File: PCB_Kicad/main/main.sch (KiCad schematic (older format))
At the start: 21 parts, among them Q1 Q_NMOS_GDS, Q2 Q_NMOS_GDS, U1 LTC3854EMSEPBF, U2 ACS70331EESATR-005U3

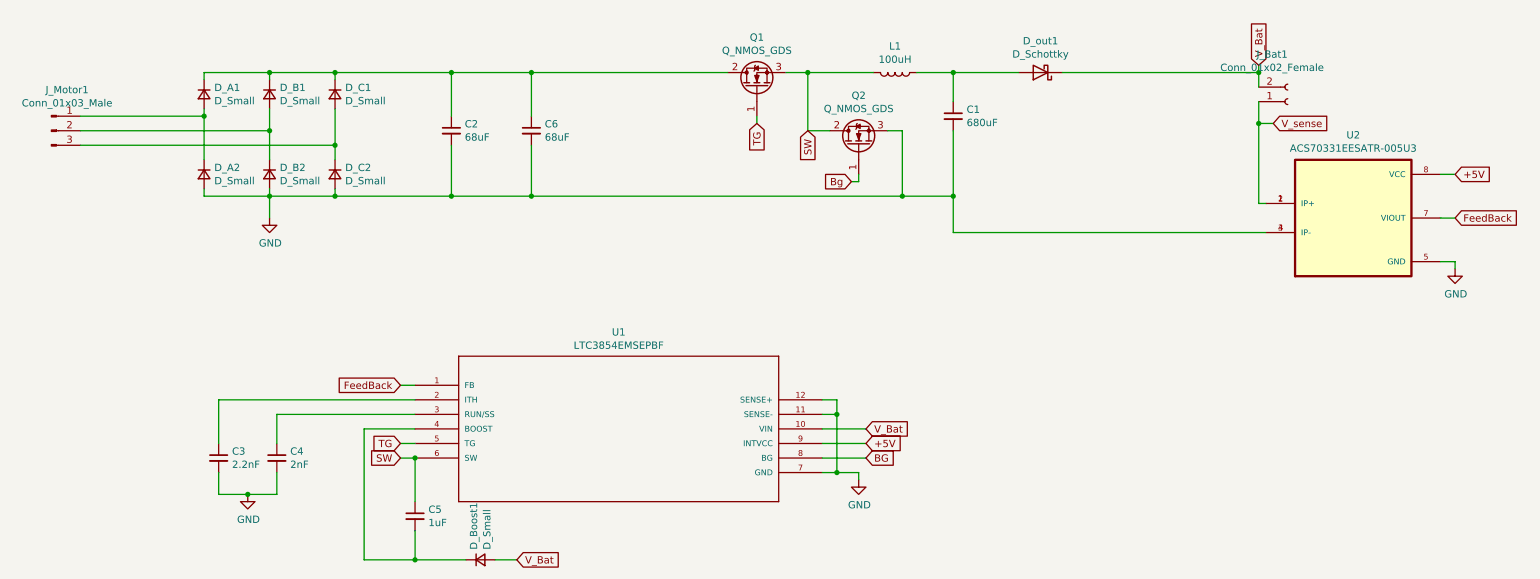
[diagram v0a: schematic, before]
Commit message: kicad update
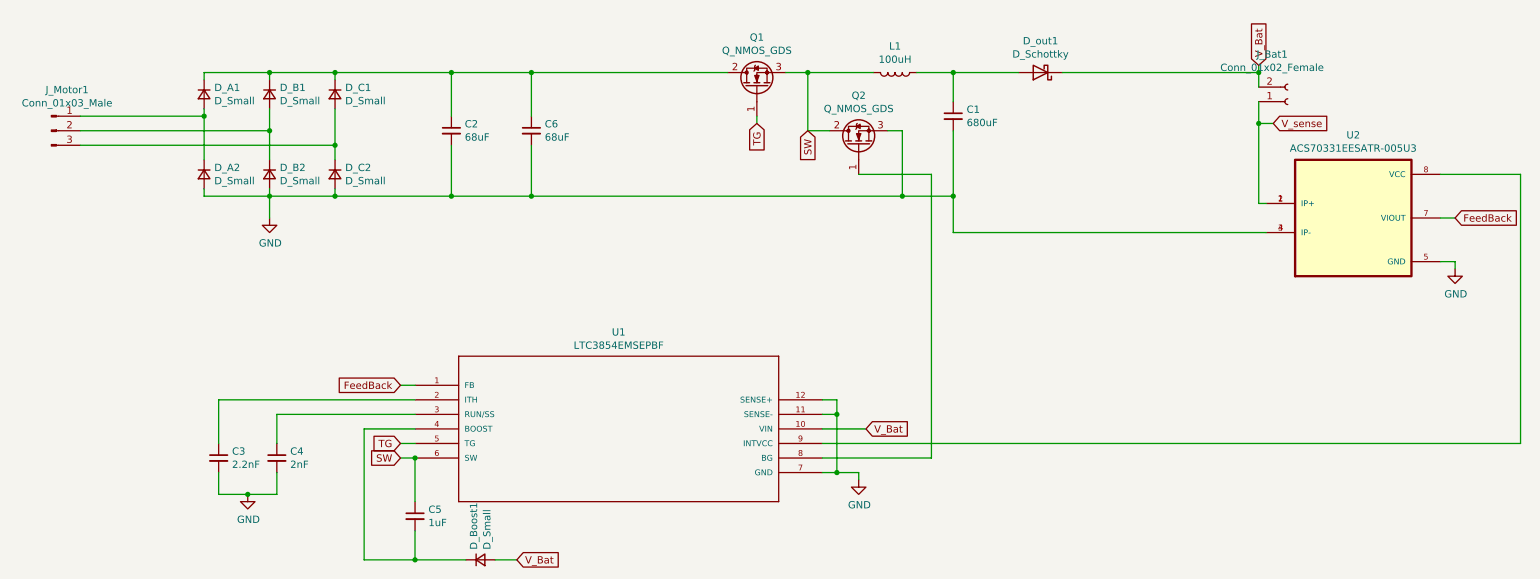
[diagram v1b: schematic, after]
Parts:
- L1: footprint Inductor_THT:L_Radial_D14.2mm_P10.00mm_Neosid_SD14 -> Inductor_SMD:L_Wuerth_HCM-1390
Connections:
- net Bg is gone; now on an unnamed net: Q2.1 (G)
- net +5V: no longer names the net of U1.9 (INTVCC), U2.8 (VCC)
- net BG: no longer names the net of U1.8 (BG)
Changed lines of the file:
@@
 F 0 "L1" V 6519 850 50  0000 C CNN
 F 1 "100uH" V 6610 850 50  0000 C CNN
-F 2 "Inductor_THT:L_Radial_D14.2mm_P10.00mm_Neosid_SD14" H 6700 850 50  0001 C CNN
+F 2 "Inductor_SMD:L_Wuerth_HCM-1390" H 6700 850 50  0001 C CNN
 F 3 "~" H 6700 850 50  0001 C CNN
 	1    6700 850
@@
 Wire Wire Line
 	10550 2150 10450 2150
-Text GLabel 10550 1550 2    50   Input ~ 0
-+5V
-Wire Wire Line
-	10450 1550 10550 1550
-Text GLabel 6500 3400 2    50   Input ~ 0
-+5V
 $Comp
 L power:GND #PWR0102
@@
 	6450 3650 6450 3600
 Wire Wire Line
-	6200 3400 6500 3400
-Wire Wire Line
 	6200 3100 6300 3100
 Wire Wire Line
@@
 Wire Wire Line
 	6500 3300 6200 3300
-Text GLabel 6500 3500 2    50   Input ~ 0
-BG
-Wire Wire Line
-	6200 3500 6500 3500
 Text GLabel 3300 3500 0    50   Input ~ 0
 SW
@@
 Wire Wire Line
 	5750 1150 5750 1200
-Text GLabel 6400 1600 0    50   Input ~ 0
-Bg
-Wire Wire Line
-	6400 1600 6450 1600
-Wire Wire Line
-	6450 1600 6450 1550
 Text GLabel 6100 1250 3    50   Input ~ 0
 SW
@@
 Wire Wire Line
 	4200 1700 6750 1700
+Wire Wire Line
+	6200 3500 6950 3500
+Wire Wire Line
+	6950 3500 6950 1550
+Wire Wire Line
+	6950 1550 6450 1550
+Wire Wire Line
+	11000 1550 11000 3400
+Wire Wire Line
+	11000 3400 6200 3400
+Wire Wire Line
+	10450 1550 11000 1550
 $EndSCHEMATC

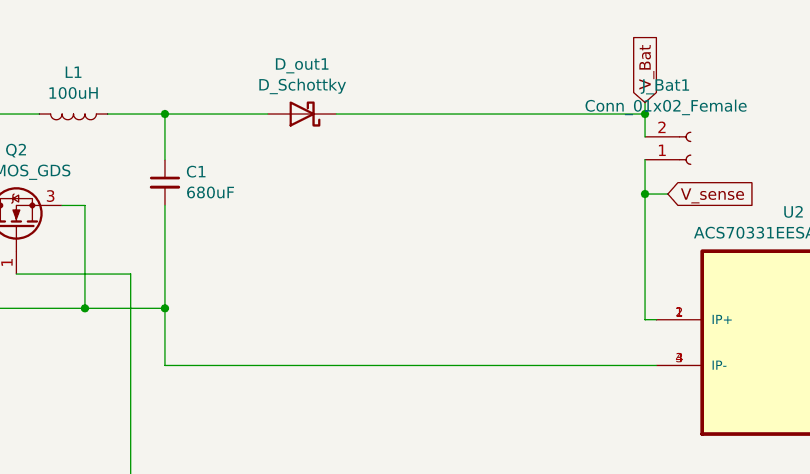
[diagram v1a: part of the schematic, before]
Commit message: model update
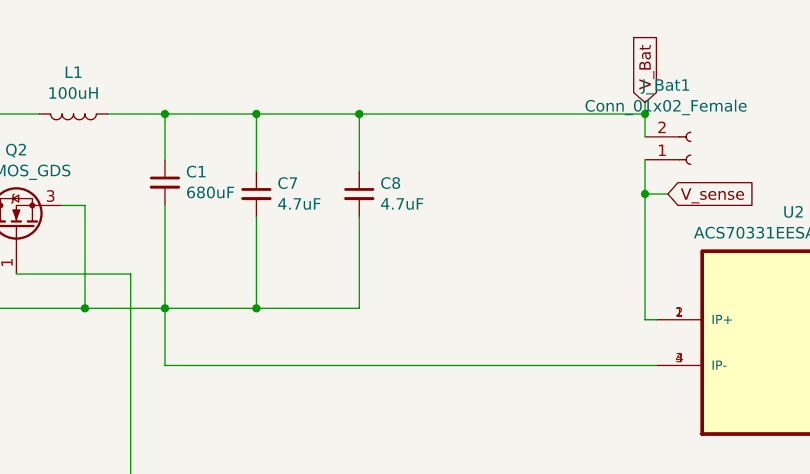
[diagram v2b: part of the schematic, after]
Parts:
- removed D_out1: D_Schottky, Diode_SMD:D_SMB, symbol Device:D_Schottky
- added C7, C8: 4.7uF, Capacitor_SMD:C_2225_5664Metric_Pad1.80x6.60mm_HandSolder, symbol Device:C_Small
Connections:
- net GND: now also C7.2, C8.2
- net V_Bat: now also C1.1, L1.1, C7.1, C8.1
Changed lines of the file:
@@
 Connection ~ 7100 850
 Wire Wire Line
-	7100 850  7550 850
+	7100 850  7500 850
 Wire Wire Line
 	7100 850  7100 1050
@@
 	9200 950  9200 850
 Wire Wire Line
-	9200 850  7850 850
-Wire Wire Line
 	9200 1050 9200 1200
 Text GLabel 9300 1200 2    50   Input ~ 0
@@
 	9200 850  9200 800
 Connection ~ 9200 850
-$Comp
-L Device:D_Schottky D_out1
-U 1 1 6006BA40
-P 7700 850
-F 0 "D_out1" H 7700 633 50  0000 C CNN
-F 1 "D_Schottky" H 7700 724 50  0000 C CNN
-F 2 "Diode_SMD:D_SMB" H 7700 850 50  0001 C CNN
-F 3 "~" H 7700 850 50  0001 C CNN
-	1    7700 850
-	-1   0    0    1
-$EndComp
 $Comp
 L power:GND #PWR0112
@@
 Wire Wire Line
 	10450 1550 11000 1550
+$Comp
+L Device:C_Small C7
+U 1 1 5FFE17AF
+P 7500 1200
+F 0 "C7" H 7592 1246 50  0000 L CNN
+F 1 "4.7uF" H 7592 1155 50  0000 L CNN
+F 2 "Capacitor_SMD:C_2225_5664Metric_Pad1.80x6.60mm_HandSolder" H 7500 1200 50  0001 C CNN
+F 3 "~" H 7500 1200 50  0001 C CNN
+	1    7500 1200
+	1    0    0    -1
+$EndComp
+Wire Wire Line
+	7500 1100 7500 850
+Connection ~ 7500 850
+Wire Wire Line
+	7500 1300 7500 1700
+Wire Wire Line
+	7500 1700 7100 1700
+Wire Wire Line
+	7500 850  7950 850
+Wire Wire Line
+	7950 1100 7950 850
+Connection ~ 7950 850
+Wire Wire Line
+	7950 1300 7950 1700
+Wire Wire Line
+	7950 1700 7500 1700
+Connection ~ 7500 1700
+$Comp
+L Device:C_Small C8
+U 1 1 5FFE1E1F
+P 7950 1200
+F 0 "C8" H 8042 1246 50  0000 L CNN
+F 1 "4.7uF" H 8042 1155 50  0000 L CNN
+F 2 "Capacitor_SMD:C_2225_5664Metric_Pad1.80x6.60mm_HandSolder" H 7950 1200 50  0001 C CNN
+F 3 "~" H 7950 1200 50  0001 C CNN
+	1    7950 1200
+	1    0    0    -1
+$EndComp
+Wire Wire Line
+	7950 850  9200 850
 $EndSCHEMATC

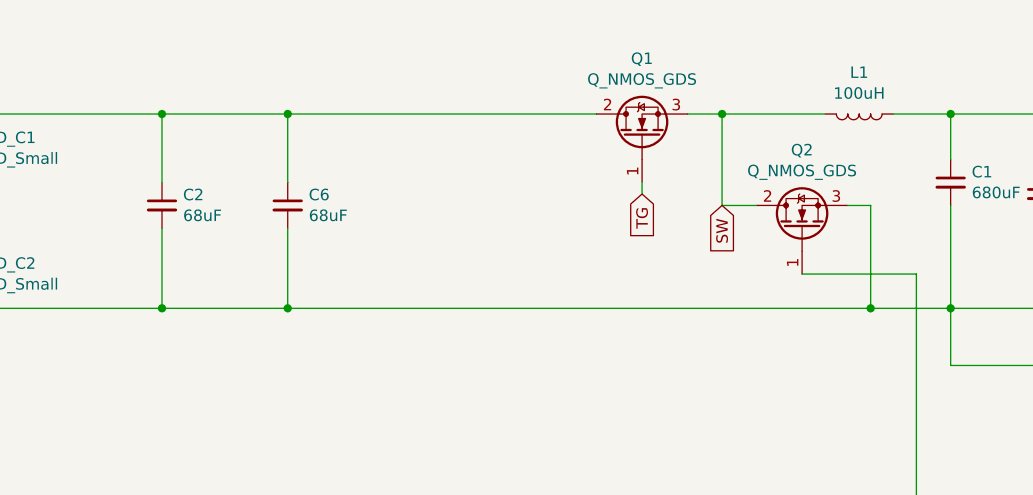
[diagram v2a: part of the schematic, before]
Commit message: kicad_updated
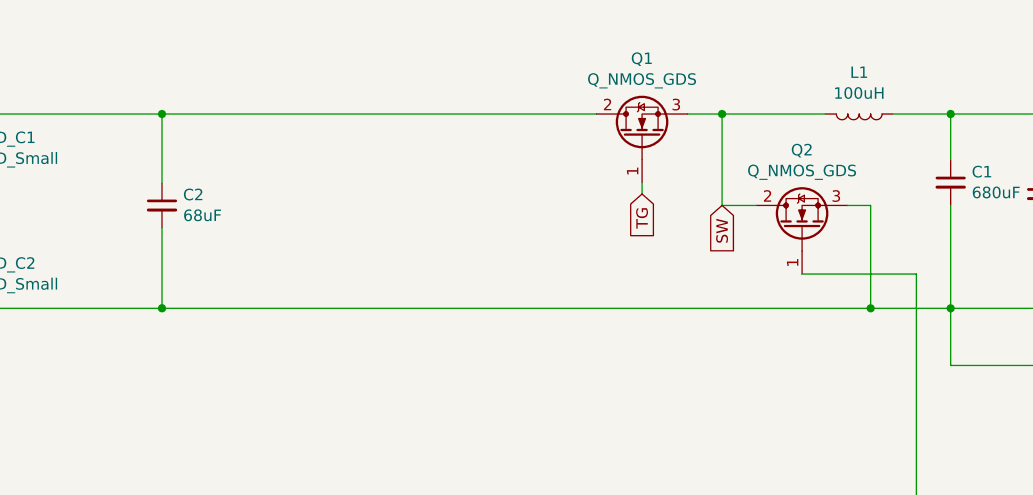
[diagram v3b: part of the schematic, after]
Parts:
- removed C6: 68uF, Capacitor_SMD:CP_Elec_6.3x7.7, symbol Device:C_Small
- C1: footprint Capacitor_SMD:CP_Elec_6.3x7.7 -> Capacitor_SMD:CP_Elec_10x7.9
- C2: footprint Capacitor_SMD:CP_Elec_6.3x7.7 -> Capacitor_THT:CP_Radial_D18.0mm_P7.50mm
- C5: footprint Capacitor_SMD:CP_Elec_6.3x7.7 -> Capacitor_SMD:CP_Elec_8x10
- C7, C8: footprint Capacitor_SMD:C_2225_5664Metric_Pad1.80x6.60mm_HandSolder -> Capacitor_SMD:C_0805_2012Metric
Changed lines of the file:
@@
 F 0 "C1" H 7192 1196 50  0000 L CNN
 F 1 "680uF" H 7192 1105 50  0000 L CNN
-F 2 "Capacitor_SMD:CP_Elec_6.3x7.7" H 7100 1150 50  0001 C CNN
+F 2 "Capacitor_SMD:CP_Elec_10x7.9" H 7100 1150 50  0001 C CNN
 F 3 "~" H 7100 1150 50  0001 C CNN
 	1    7100 1150
@@
 F 0 "C2" H 3742 1296 50  0000 L CNN
 F 1 "68uF" H 3742 1205 50  0000 L CNN
-F 2 "Capacitor_SMD:CP_Elec_6.3x7.7" H 3650 1250 50  0001 C CNN
+F 2 "Capacitor_THT:CP_Radial_D18.0mm_P7.50mm" H 3650 1250 50  0001 C CNN
 F 3 "~" H 3650 1250 50  0001 C CNN
 	1    3650 1250
@@
 	0    -1   -1   0
 $EndComp
-Wire Wire Line
-	3650 1700 4200 1700
 Wire Wire Line
 	5950 850  6100 850
@@
 F 0 "C5" H 3492 3946 50  0000 L CNN
 F 1 "1uF" H 3492 3855 50  0000 L CNN
-F 2 "Capacitor_SMD:CP_Elec_6.3x7.7" H 3400 3900 50  0001 C CNN
+F 2 "Capacitor_SMD:CP_Elec_8x10" H 3400 3900 50  0001 C CNN
 F 3 "~" H 3400 3900 50  0001 C CNN
 	1    3400 3900
@@
 Wire Wire Line
 	3400 4200 3050 4200
-$Comp
-L Device:C_Small C6
-U 1 1 5FF1C9C9
-P 4200 1250
-F 0 "C6" H 4292 1296 50  0000 L CNN
-F 1 "68uF" H 4292 1205 50  0000 L CNN
-F 2 "Capacitor_SMD:CP_Elec_6.3x7.7" H 4200 1250 50  0001 C CNN
-F 3 "~" H 4200 1250 50  0001 C CNN
-	1    4200 1250
-	1    0    0    -1
-$EndComp
-Wire Wire Line
-	4200 1150 4200 850
-Wire Wire Line
-	3650 850  4200 850
-Connection ~ 4200 850
-Wire Wire Line
-	4200 850  5550 850
-Wire Wire Line
-	4200 1350 4200 1700
-Connection ~ 4200 1700
-Wire Wire Line
-	4200 1700 6750 1700
 Wire Wire Line
 	6200 3500 6950 3500
@@
 F 0 "C7" H 7592 1246 50  0000 L CNN
 F 1 "4.7uF" H 7592 1155 50  0000 L CNN
-F 2 "Capacitor_SMD:C_2225_5664Metric_Pad1.80x6.60mm_HandSolder" H 7500 1200 50  0001 C CNN
+F 2 "Capacitor_SMD:C_0805_2012Metric" H 7500 1200 50  0001 C CNN
 F 3 "~" H 7500 1200 50  0001 C CNN
 	1    7500 1200
@@
 F 0 "C8" H 8042 1246 50  0000 L CNN
 F 1 "4.7uF" H 8042 1155 50  0000 L CNN
-F 2 "Capacitor_SMD:C_2225_5664Metric_Pad1.80x6.60mm_HandSolder" H 7950 1200 50  0001 C CNN
+F 2 "Capacitor_SMD:C_0805_2012Metric" H 7950 1200 50  0001 C CNN
 F 3 "~" H 7950 1200 50  0001 C CNN
 	1    7950 1200
@@
 Wire Wire Line
 	7950 850  9200 850
+Wire Wire Line
+	3650 850  5550 850
+Wire Wire Line
+	3650 1700 6750 1700
 $EndSCHEMATC
